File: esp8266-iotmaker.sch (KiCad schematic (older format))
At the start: 72 parts, among them J1 CONN_01X04, J2 CONN_01X02, J3 CONN_01X08, J4 CONN_01X06, J5 CONN_01X08, J6 CONN_01X04, Q1 S8050, Q2 S8050, SW1 SW_Push, SW2 SW_Push, U1 usb_mini_b, U2 chip-esp8266, U3 CP2102, U4 25Q32, U5 mcp73831, U6 AMS1117-3.3, U7 AMS1117-3.3, U8 MOSFET-P, Y1 26MHz

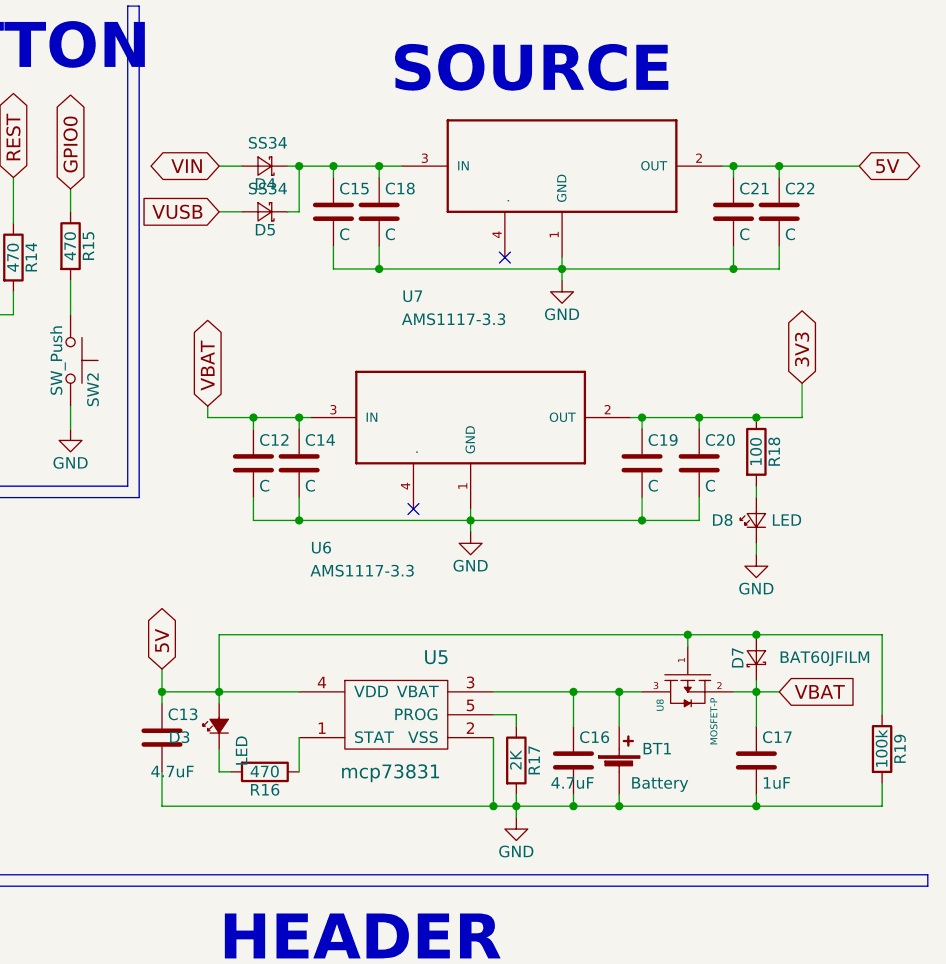
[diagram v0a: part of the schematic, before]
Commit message: complete pcb source
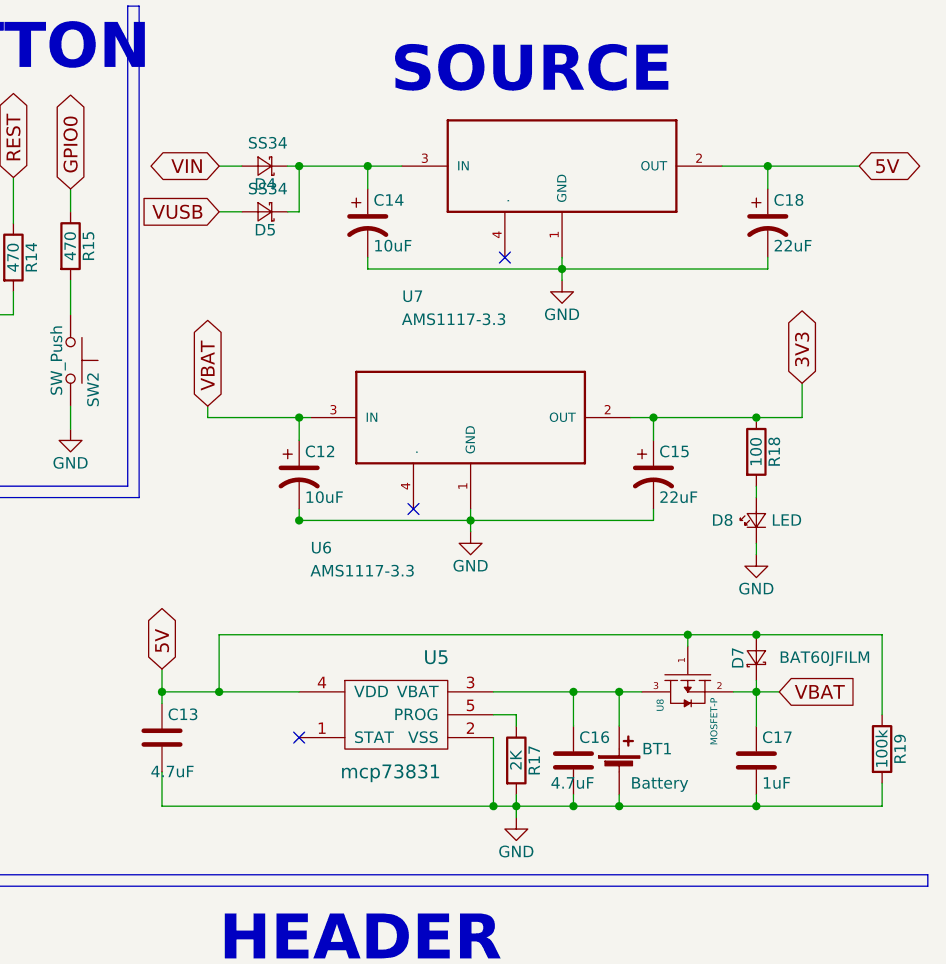
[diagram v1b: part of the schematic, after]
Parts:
- removed C12, C14, C15, C18, C19, C20, C21, C22: C, esp8266:C_0603, symbol C
- removed D3: LED, LEDs:LED_0603, symbol LED_Small_ALT
- removed R16: 470, esp8266:R_0603, symbol R
- added C12, C14: 10uF, Capacitors_SMD:CP_Elec_4x5.3, symbol CP1
- added C15, C18: 22uF, Capacitors_SMD:CP_Elec_4x5.3, symbol CP1
- D7: footprint Diodes_SMD:D_SOD-123 -> Diodes_SMD:D_SOD-323
- SW1, SW2: footprint esp8266:Tact_Switch_TS6X3.6 -> esp8266:micro-buttom
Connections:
- net 3V3: now also C15.1
- net 5V: now also C18.1
- net GND: now also C12.2, C14.2, C15.2, C18.2
- net VBAT: now also C12.1
- net at D4.1 (K), D5.1 (K), U7.3 (IN): now also C14.1
- no-connect marks 22 -> 23
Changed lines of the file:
@@
 F 0 "SW1" H 6950 2150 50  0000 L CNN
 F 1 "SW_Push" H 6900 1990 50  0000 C CNN
-F 2 "esp8266:Tact_Switch_TS6X3.6" H 6900 2250 50  0001 C CNN
+F 2 "esp8266:micro-buttom" H 6900 2250 50  0001 C CNN
 F 3 "" H 6900 2250 50  0001 C CNN
 	1    6900 2050
@@
 F 0 "SW2" H 7550 2100 50  0000 L CNN
 F 1 "SW_Push" H 7500 1940 50  0000 C CNN
-F 2 "esp8266:Tact_Switch_TS6X3.6" H 7500 2200 50  0001 C CNN
+F 2 "esp8266:micro-buttom" H 7500 2200 50  0001 C CNN
 F 3 "" H 7500 2200 50  0001 C CNN
 	1    7500 2000
@@
 VBAT
 $Comp
-L mcp73831 U5
-U 1 1 59F0B81A
-P 9000 3700
-F 0 "U5" H 9100 4100 60  0000 C CNN
-F 1 "mcp73831" H 8900 3600 60  0000 C CNN
-F 2 "TO_SOT_Packages_SMD:SOT-23-5" H 9000 3700 60  0001 C CNN
-F 3 "" H 9000 3700 60  0001 C CNN
-	1    9000 3700
-	1    0    0    -1
-$EndComp
-$Comp
 L R R17
 U 1 1 59F0BAE6
@@
 F 0 "D7" H 10450 3380 50  0000 L CNN
 F 1 "BAT60JFILM" V 10500 2800 50  0000 L CNN
-F 2 "Diodes_SMD:D_SOD-123" V 10500 3300 50  0001 C CNN
+F 2 "Diodes_SMD:D_SOD-323" V 10500 3300 50  0001 C CNN
 F 3 "" V 10500 3300 50  0001 C CNN
 	1    10500 3300
@@
 Text GLabel 10600 3450 2    60   Input ~ 0
 VBAT
-$Comp
-L LED_Small_ALT D3
-U 1 1 59F1B94D
-P 8150 3600
-F 0 "D3" V 8100 3725 50  0000 L CNN
-F 1 "LED" H 7975 3500 50  0000 L CNN
-F 2 "LEDs:LED_0603" V 8150 3600 50  0001 C CNN
-F 3 "" V 8150 3600 50  0001 C CNN
-	1    8150 3600
-	0    -1   -1   0
-$EndComp
-$Comp
-L R R16
-U 1 1 59F1BAA4
-P 8350 3800
-F 0 "R16" V 8430 3800 50  0000 C CNN
-F 1 "470" V 8350 3800 50  0000 C CNN
-F 2 "esp8266:R_0603" V 8280 3800 50  0001 C CNN
-F 3 "" H 8350 3800 50  0001 C CNN
-	1    8350 3800
-	0    1    1    0
-$EndComp
 $Comp
 L LED_Small D8
@@
 Text Notes 7550 5950 0    60   ~ 0
 ADC IN
-$Comp
-L C C18
-U 1 1 59F5AC27
-P 8850 1350
-F 0 "C18" H 8875 1450 50  0000 L CNN
-F 1 "C" H 8875 1250 50  0000 L CNN
-F 2 "esp8266:C_0603" H 8888 1200 50  0001 C CNN
-F 3 "" H 8850 1350 50  0001 C CNN
-	1    8850 1350
-	1    0    0    -1
-$EndComp
-$Comp
-L C C15
-U 1 1 59F5ACC4
-P 8650 1350
-F 0 "C15" H 8675 1450 50  0000 L CNN
-F 1 "C" H 8675 1250 50  0000 L CNN
-F 2 "esp8266:C_0603" H 8688 1200 50  0001 C CNN
-F 3 "" H 8650 1350 50  0001 C CNN
-	1    8650 1350
-	1    0    0    -1
-$EndComp
-$Comp
-L C C21
-U 1 1 59F5B90C
-P 10400 1350
-F 0 "C21" H 10425 1450 50  0000 L CNN
-F 1 "C" H 10425 1250 50  0000 L CNN
-F 2 "esp8266:C_0603" H 10438 1200 50  0001 C CNN
-F 3 "" H 10400 1350 50  0001 C CNN
-	1    10400 1350
-	1    0    0    -1
-$EndComp
-$Comp
-L C C22
-U 1 1 59F5B9AB
-P 10600 1350
-F 0 "C22" H 10625 1450 50  0000 L CNN
-F 1 "C" H 10625 1250 50  0000 L CNN
-F 2 "esp8266:C_0603" H 10638 1200 50  0001 C CNN
-F 3 "" H 10600 1350 50  0001 C CNN
-	1    10600 1350
-	1    0    0    -1
-$EndComp
-$Comp
-L C C14
-U 1 1 59F5C166
-P 8500 2450
-F 0 "C14" H 8525 2550 50  0000 L CNN
-F 1 "C" H 8525 2350 50  0000 L CNN
-F 2 "esp8266:C_0603" H 8538 2300 50  0001 C CNN
-F 3 "" H 8500 2450 50  0001 C CNN
-	1    8500 2450
-	1    0    0    -1
-$EndComp
-$Comp
-L C C12
-U 1 1 59F5C207
-P 8300 2450
-F 0 "C12" H 8325 2550 50  0000 L CNN
-F 1 "C" H 8325 2350 50  0000 L CNN
-F 2 "esp8266:C_0603" H 8338 2300 50  0001 C CNN
-F 3 "" H 8300 2450 50  0001 C CNN
-	1    8300 2450
-	1    0    0    -1
-$EndComp
-$Comp
-L C C20
-U 1 1 59F5CDA6
-P 10250 2450
-F 0 "C20" H 10275 2550 50  0000 L CNN
-F 1 "C" H 10275 2350 50  0000 L CNN
-F 2 "esp8266:C_0603" H 10288 2300 50  0001 C CNN
-F 3 "" H 10250 2450 50  0001 C CNN
-	1    10250 2450
-	1    0    0    -1
-$EndComp
-$Comp
-L C C19
-U 1 1 59F5D11F
-P 10000 2450
-F 0 "C19" H 10025 2550 50  0000 L CNN
-F 1 "C" H 10025 2350 50  0000 L CNN
-F 2 "esp8266:C_0603" H 10038 2300 50  0001 C CNN
-F 3 "" H 10000 2450 50  0001 C CNN
-	1    10000 2450
-	1    0    0    -1
-$EndComp
 Wire Wire Line
 	7500 1650 7500 1800
@@
 Wire Wire Line
 	9650 1550 9650 1650
-Wire Wire Line
-	8650 1600 10600 1600
-Wire Wire Line
-	8850 1600 8850 1500
 Connection ~ 9650 1600
-Wire Wire Line
-	10400 1600 10400 1500
-Wire Wire Line
-	10400 1200 10400 1150
-Connection ~ 10400 1150
-Connection ~ 8850 1150
 Wire Wire Line
 	3800 3000 3650 3000
@@
 Wire Wire Line
 	9250 2650 9250 2750
-Wire Wire Line
-	8300 2700 10250 2700
-Wire Wire Line
-	8500 2700 8500 2600
 Connection ~ 9250 2700
 Wire Wire Line
-	10000 2700 10000 2600
-Wire Wire Line
-	10000 2300 10000 2250
-Wire Wire Line
 	9950 2250 10700 2250
-Connection ~ 10000 2250
 Wire Wire Line
 	10700 2250 10700 2100
-Connection ~ 10250 2250
 Wire Wire Line
 	8100 2250 8550 2250
@@
 Connection ~ 9700 3450
 Wire Wire Line
-	8500 2250 8500 2300
+	8500 2250 8500 2350
 Connection ~ 8500 2250
-Wire Wire Line
-	8850 1150 8850 1200
 Connection ~ 7900 3450
 Wire Wire Line
@@
 Wire Wire Line
 	10400 3450 10600 3450
-Wire Wire Line
-	8150 3200 8150 3500
 Wire Wire Line
 	8150 3200 11050 3200
@@
 	11050 3950 11050 3850
 Connection ~ 10500 3950
-Wire Wire Line
-	8150 3700 8150 3800
-Wire Wire Line
-	8150 3800 8200 3800
-Wire Wire Line
-	8500 3650 8500 3800
 Wire Bus Line
 	5600 2550 5600 4250
@@
 Wire Wire Line
 	10650 4900 10600 4900
-Wire Wire Line
-	8650 1200 8650 1150
-Connection ~ 8650 1150
-Wire Wire Line
-	8650 1500 8650 1600
-Connection ~ 8850 1600
-Wire Wire Line
-	10600 1200 10600 1150
-Connection ~ 10600 1150
-Wire Wire Line
-	10600 1600 10600 1500
-Connection ~ 10400 1600
 Connection ~ 10500 2250
 Wire Wire Line
-	10250 2300 10250 2250
-Wire Wire Line
-	10250 2700 10250 2600
-Connection ~ 10000 2700
-Wire Wire Line
-	8300 2300 8300 2250
-Connection ~ 8300 2250
-Wire Wire Line
-	8300 2600 8300 2700
+	9900 5900 9450 5900
+Wire Wire Line
+	9800 5100 9800 5150
+$Comp
+L CP1 C12
+U 1 1 59F9F26A
+P 8500 2500
+F 0 "C12" H 8525 2600 50  0000 L CNN
+F 1 "10uF" H 8525 2400 50  0000 L CNN
+F 2 "Capacitors_SMD:CP_Elec_4x5.3" H 8500 2500 50  0001 C CNN
+F 3 "" H 8500 2500 50  0001 C CNN
+	1    8500 2500
+	1    0    0    -1
+$EndComp
+Wire Wire Line
+	8500 2650 8500 2700
 Connection ~ 8500 2700
 Wire Wire Line
-	9900 5900 9450 5900
-Wire Wire Line
-	9800 5100 9800 5150
+	8500 2700 10050 2700
+$Comp
+L CP1 C15
+U 1 1 59F9FDF4
+P 10050 2500
+F 0 "C15" H 10075 2600 50  0000 L CNN
+F 1 "22uF" H 10075 2400 50  0000 L CNN
+F 2 "Capacitors_SMD:CP_Elec_4x5.3" H 10050 2500 50  0001 C CNN
+F 3 "" H 10050 2500 50  0001 C CNN
+	1    10050 2500
+	1    0    0    -1
+$EndComp
+Wire Wire Line
+	10050 2350 10050 2250
+Connection ~ 10050 2250
+Wire Wire Line
+	10050 2700 10050 2650
+$Comp
+L CP1 C18
+U 1 1 59FA0E70
+P 10550 1400
+F 0 "C18" H 10575 1500 50  0000 L CNN
+F 1 "22uF" H 10575 1300 50  0000 L CNN
+F 2 "Capacitors_SMD:CP_Elec_4x5.3" H 10550 1400 50  0001 C CNN
+F 3 "" H 10550 1400 50  0001 C CNN
+	1    10550 1400
+	1    0    0    -1
+$EndComp
+$Comp
+L CP1 C14
+U 1 1 59FA0F68
+P 8800 1400
+F 0 "C14" H 8825 1500 50  0000 L CNN
+F 1 "10uF" H 8825 1300 50  0000 L CNN
+F 2 "Capacitors_SMD:CP_Elec_4x5.3" H 8800 1400 50  0001 C CNN
+F 3 "" H 8800 1400 50  0001 C CNN
+	1    8800 1400
+	1    0    0    -1
+$EndComp
+Wire Wire Line
+	8800 1250 8800 1150
+Connection ~ 8800 1150
+Wire Wire Line
+	8800 1550 8800 1600
+Wire Wire Line
+	8800 1600 10550 1600
+Wire Wire Line
+	10550 1600 10550 1550
+Wire Wire Line
+	10550 1250 10550 1150
+Connection ~ 10550 1150
+Wire Wire Line
+	8150 3450 8150 3200
+$Comp
+L mcp73831 U5
+U 1 1 59F0B81A
+P 9000 3700
+F 0 "U5" H 9100 4100 60  0000 C CNN
+F 1 "mcp73831" H 8900 3600 60  0000 C CNN
+F 2 "TO_SOT_Packages_SMD:SOT-23-5" H 9000 3700 60  0001 C CNN
+F 3 "" H 9000 3700 60  0001 C CNN
+	1    9000 3700
+	1    0    0    -1
+$EndComp
+NoConn ~ 8500 3650
 $EndSCHEMATC
